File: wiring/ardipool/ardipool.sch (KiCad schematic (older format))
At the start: 23 parts, among them K1 filter, K2 ph, P1 Digital, P10 CONN_01X01, P11 CONN_01X01, P12 CONN_01X01, P13 CONN_01X01, P2 Power, P3 Analog, P4 Analog, P5 PWM, P6 PWM, P7 Communication, P8 CONN_01X01, P9 CONN_01X01, SW1 SW_Push_Dual, U1 DS18B20, U2 DS18B20, U3 DHT11, U4 DS1307+

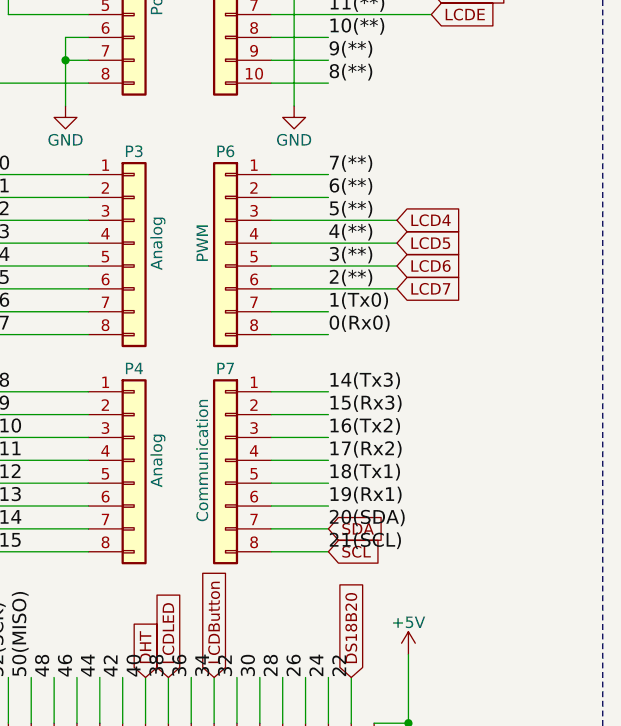
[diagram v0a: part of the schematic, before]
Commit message: schem
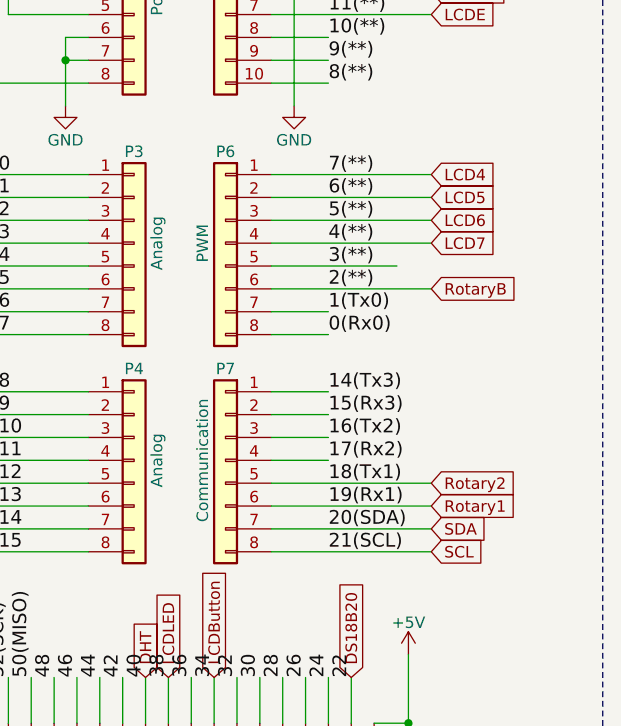
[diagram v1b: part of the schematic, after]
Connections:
- net 6(**) is gone; now on net LCD5: P6.2 (Pin_2)
- net 7(**) is gone; now on net LCD4: P6.1 (Pin_1)
- net LCD4: no longer P6.3 (Pin_3)
- net LCD5: no longer P6.4 (Pin_4)
- net LCD6: now also P6.3 (Pin_3); no longer P6.5 (Pin_5)
- net LCD7: now also P6.4 (Pin_4); no longer P6.6 (Pin_6)
- net 18(Tx1) renamed Rotary2
- net 19(Rx1) renamed Rotary1
- new net 3(**): P6.5 (Pin_5)
- new net RotaryB: P6.6 (Pin_6)
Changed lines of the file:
@@
 	8900 3150 9350 3150
 Wire Wire Line
-	10400 2450 10150 2450
-Wire Wire Line
-	10150 2550 10400 2550
-Wire Wire Line
 	10400 3050 10150 3050
 Wire Wire Line
@@
 Wire Wire Line
 	10150 3700 10400 3700
-Wire Wire Line
-	10400 3800 10150 3800
-Wire Wire Line
-	10150 3900 10400 3900
-Wire Wire Line
-	10400 4000 10150 4000
-Wire Wire Line
-	10150 4100 10400 4100
 Wire Wire Line
 	10500 4850 10500 4650
@@
 	1    0    0    -1
 $EndComp
-Text GLabel 10400 4000 2    50   Input ~ 0
+Text GLabel 10850 4000 2    50   Input ~ 0
 SDA
-Text GLabel 10400 4100 2    50   Input ~ 0
+Text GLabel 10850 4100 2    50   Input ~ 0
 SCL
 Wire Wire Line
@@
 Wire Wire Line
 	6050 5850 6300 5850
-Text GLabel 10700 2650 2    50   Input ~ 0
+Text GLabel 10850 2450 2    50   Input ~ 0
 LCD4
-Text GLabel 10700 2750 2    50   Input ~ 0
+Text GLabel 10850 2550 2    50   Input ~ 0
 LCD5
-Text GLabel 10700 2850 2    50   Input ~ 0
+Text GLabel 10850 2650 2    50   Input ~ 0
 LCD6
-Text GLabel 10700 2950 2    50   Input ~ 0
+Text GLabel 10850 2750 2    50   Input ~ 0
 LCD7
 Wire Wire Line
-	10150 2650 10700 2650
-Wire Wire Line
-	10150 2750 10700 2750
-Wire Wire Line
 	10150 2850 10700 2850
-Wire Wire Line
-	10150 2950 10700 2950
 Text GLabel 10850 1650 2    50   Input ~ 0
 LCDRS
@@
 Wire Wire Line
 	3250 4000 3250 3900
+Wire Wire Line
+	10150 2450 10850 2450
+Wire Wire Line
+	10150 2550 10850 2550
+Wire Wire Line
+	10150 2650 10850 2650
+Wire Wire Line
+	10150 2750 10850 2750
+Wire Wire Line
+	10150 4000 10850 4000
+Wire Wire Line
+	10150 4100 10850 4100
+Text GLabel 10850 3900 2    50   Input ~ 0
+Rotary1
+Text GLabel 10850 3800 2    50   Input ~ 0
+Rotary2
+Text GLabel 10850 2950 2    50   Input ~ 0
+RotaryB
+Wire Wire Line
+	10150 2950 10850 2950
+Wire Wire Line
+	10150 3800 10850 3800
+Wire Wire Line
+	10150 3900 10850 3900
 $EndSCHEMATC
